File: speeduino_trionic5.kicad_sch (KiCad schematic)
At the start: 3 parts, among them U1 Olimex_STM32-407_Extension_He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

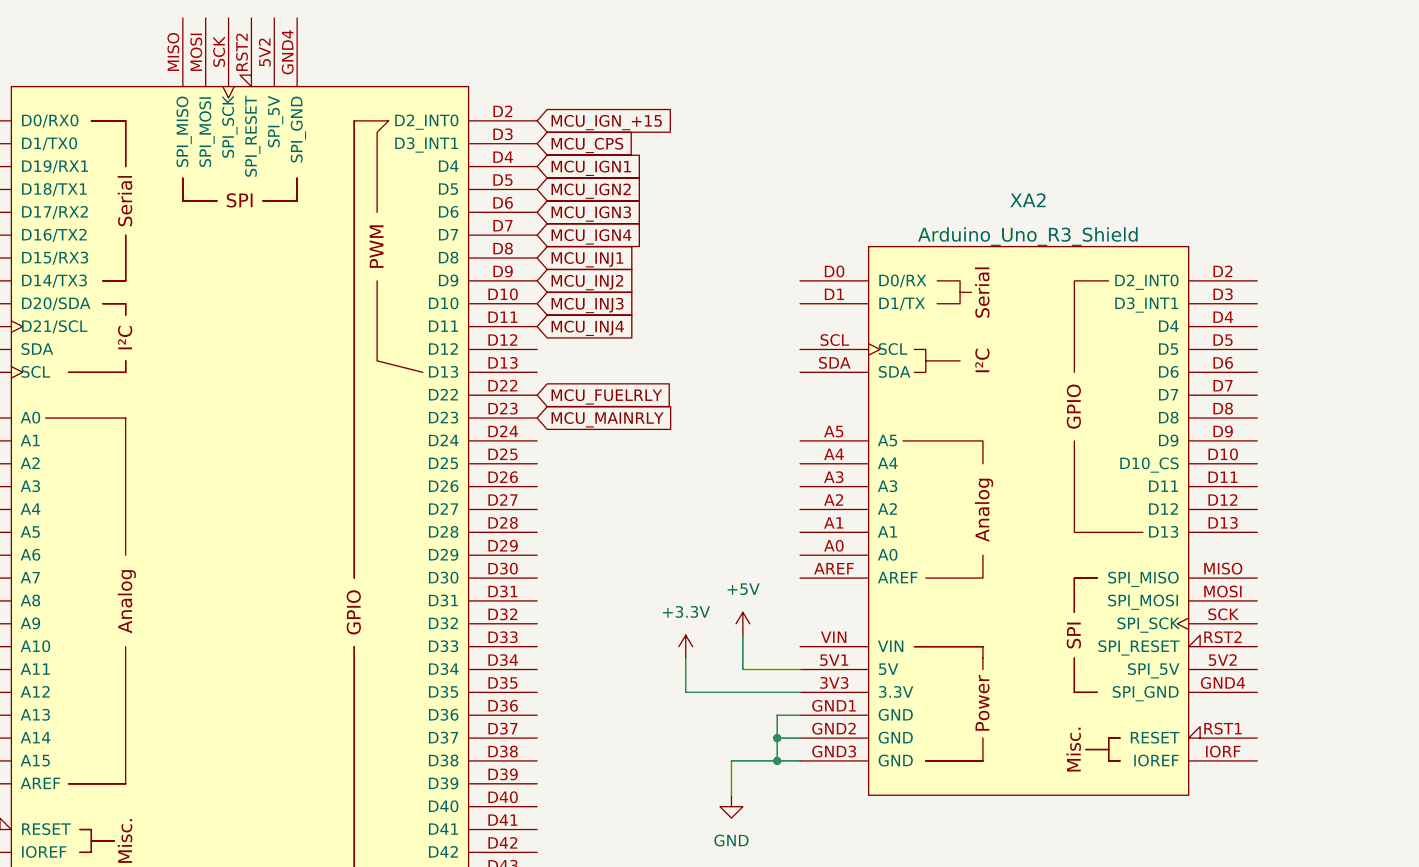
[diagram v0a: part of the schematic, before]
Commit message: Add stuff
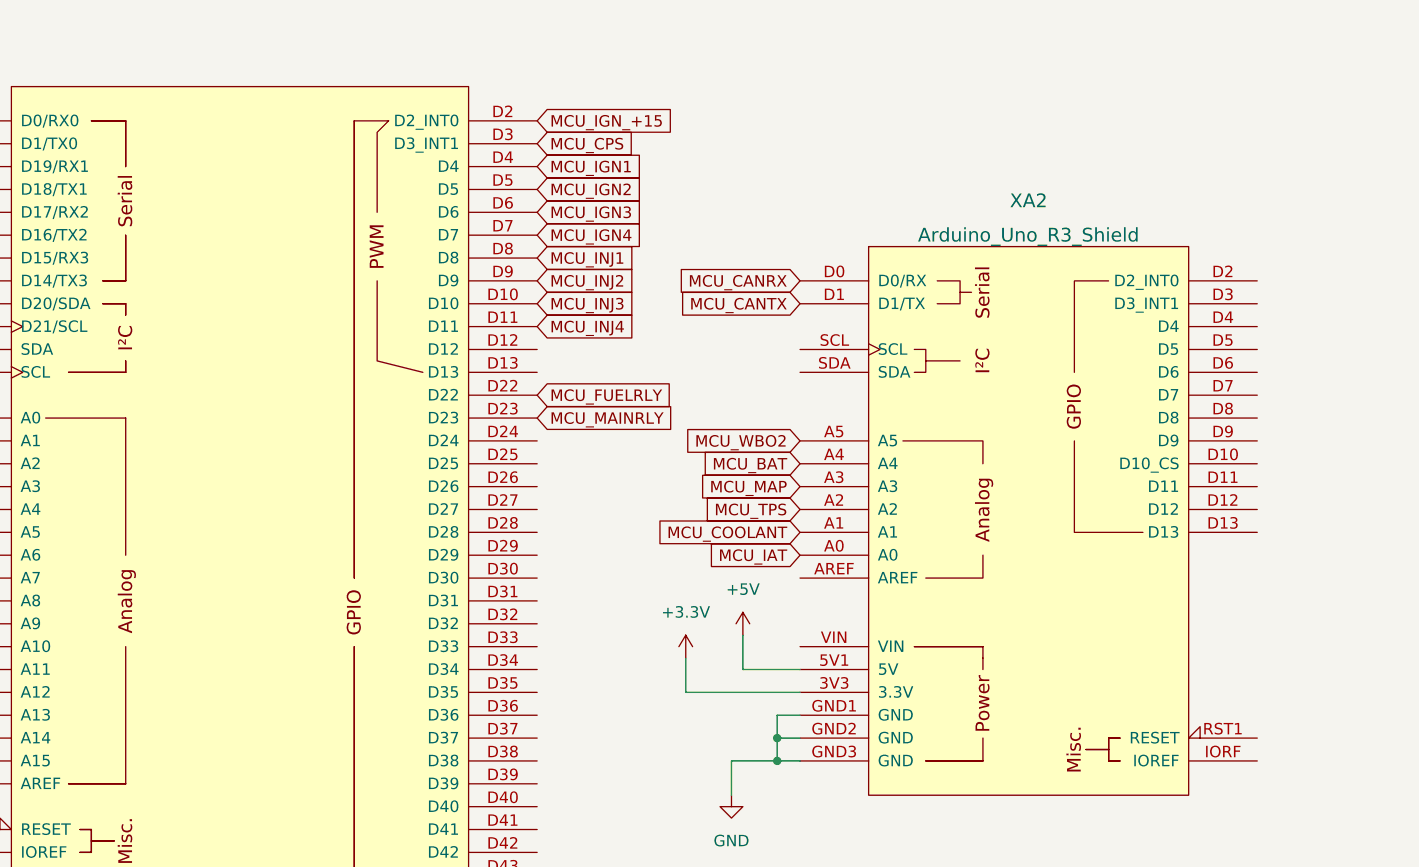
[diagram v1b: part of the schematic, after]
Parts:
- XA1: footprint PCM_arduino-library:Arduino_Mega2560_Shield -> arduino-library:Arduino_Mega2560_Shield
- XA2: footprint PCM_arduino-library:Arduino_Uno_R3_Shield -> arduino-library:Arduino_Uno_R3_Shield
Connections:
- net MCU_BAT: now also XA2.A4
- net MCU_COOLANT: now also XA2.A1
- net MCU_IAT: now also XA2.A0
- net MCU_MAP: now also XA2.A3
- net MCU_TPS: now also XA2.A2
- net MCU_WBO2: now also XA2.A5
- net MCU_CANRX: now reaches XA2.D0 (D0/RX)
- net MCU_CANTX: now reaches XA2.D1 (D1/TX)
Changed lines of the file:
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@@
     (stroke (width 0) (type default) (color 0 0 0 0))
   )
+  (global_label "MCU_MAP" (shape input) (at 129.54 76.2 180) (fields_autoplaced)
+    (effects (font (size 1.27 1.27)) (justify right))
+    (property "Intersheet References" "${INTERSHEET_REFS}" (id 0) (at 118.3863 76.1206 0)
+      (effects (font (size 1.27 1.27)) (justify right) hide)
+    )
+  )
+  (global_label "MCU_BAT" (shape input) (at 129.54 73.66 180) (fields_autoplaced)
+    (effects (font (size 1.27 1.27)) (justify right))
+    (property "Intersheet References" "${INTERSHEET_REFS}" (id 0) (at 118.8701 73.5806 0)
+      (effects (font (size 1.27 1.27)) (justify right) hide)
+    )
+  )
+  (global_label "MCU_CANTX" (shape input) (at 129.54 55.88 180) (fields_autoplaced)
+    (effects (font (size 1.27 1.27)) (justify right))
+    (property "Intersheet References" "${INTERSHEET_REFS}" (id 0) (at 116.3301 55.8006 0)
+      (effects (font (size 1.27 1.27)) (justify right) hide)
+    )
+  )
   (global_label "MCU_INJ3" (shape input) (at 100.33 55.88 0) (fields_autoplaced)
     (effects (font (size 1.27 1.27)) (justify left))
@@
     )
   )
+  (global_label "MCU_TPS" (shape input) (at 129.54 78.74 180) (fields_autoplaced)
+    (effects (font (size 1.27 1.27)) (justify right))
+    (property "Intersheet References" "${INTERSHEET_REFS}" (id 0) (at 118.7491 78.6606 0)
+      (effects (font (size 1.27 1.27)) (justify right) hide)
+    )
+  )
+  (global_label "MCU_CANRX" (shape input) (at 129.54 53.34 180) (fields_autoplaced)
+    (effects (font (size 1.27 1.27)) (justify right))
+    (property "Intersheet References" "${INTERSHEET_REFS}" (id 0) (at 116.0277 53.2606 0)
+      (effects (font (size 1.27 1.27)) (justify right) hide)
+    )
+  )
+  (global_label "MCU_IAT" (shape input) (at 129.54 83.82 180) (fields_autoplaced)
+    (effects (font (size 1.27 1.27)) (justify right))
+    (property "Intersheet References" "${INTERSHEET_REFS}" (id 0) (at 119.5353 83.7406 0)
+      (effects (font (size 1.27 1.27)) (justify right) hide)
+    )
+  )
   (global_label "MCU_INJ4" (shape input) (at 100.33 58.42 0) (fields_autoplaced)
     (effects (font (size 1.27 1.27)) (justify left))
@@
     )
   )
+  (global_label "MCU_WBO2" (shape input) (at 129.54 71.12 180) (fields_autoplaced)
+    (effects (font (size 1.27 1.27)) (justify right))
+    (property "Intersheet References" "${INTERSHEET_REFS}" (id 0) (at 116.9348 71.0406 0)
+      (effects (font (size 1.27 1.27)) (justify right) hide)
+    )
+  )
   (global_label "MCU_MAINRLY" (shape input) (at 100.33 68.58 0) (fields_autoplaced)
     (effects (font (size 1.27 1.27)) (justify left))
@@
     (property "Intersheet References" "${INTERSHEET_REFS}" (id 0) (at 112.0885 43.1006 0)
       (effects (font (size 1.27 1.27)) (justify left) hide)
+    )
+  )
+  (global_label "MCU_COOLANT" (shape input) (at 129.54 81.28 180) (fields_autoplaced)
+    (effects (font (size 1.27 1.27)) (justify right))
+    (property "Intersheet References" "${INTERSHEET_REFS}" (id 0) (at 113.8506 81.2006 0)
+      (effects (font (size 1.27 1.27)) (justify right) hide)
     )
   )
@@
       (effects (font (size 1.524 1.524)))
     )
-    (property "Footprint" "PCM_arduino-library:Arduino_Mega2560_Shield" (id 2) (at 67.31 163.83 0)
+    (property "Footprint" "arduino-library:Arduino_Mega2560_Shield" (id 2) (at 67.31 163.83 0)
       (effects (font (size 1.524 1.524)) hide)
     )
@@
     (pin "3V3")
     (pin "5V1")
-    (pin "5V2")
     (pin "5V3")
     (pin "5V4")
@@
     (pin "GND2")
     (pin "GND3")
-    (pin "GND4")
     (pin "GND5")
     (pin "GND6")
     (pin "IORF")
-    (pin "MISO")
-    (pin "MOSI")
     (pin "RST1")
-    (pin "RST2")
-    (pin "SCK")
     (pin "SCL")
     (pin "SDA")
@@
       (effects (font (size 1.524 1.524)))
     )
-    (property "Footprint" "PCM_arduino-library:Arduino_Uno_R3_Shield" (id 2) (at 154.94 118.11 0)
+    (property "Footprint" "arduino-library:Arduino_Uno_R3_Shield" (id 2) (at 154.94 118.11 0)
       (effects (font (size 1.524 1.524)) hide)
     )
@@
     (pin "3V3")
     (pin "5V1")
-    (pin "5V2")
     (pin "A0")
     (pin "A1")
@@
     (pin "GND2")
     (pin "GND3")
-    (pin "GND4")
     (pin "IORF")
-    (pin "MISO")
-    (pin "MOSI")
     (pin "RST1")
-    (pin "RST2")
-    (pin "SCK")
     (pin "SCL")
     (pin "SDA")
@@
       (reference "#PWR0160") (unit 1) (value "+3.3V") (footprint "")
     )
+    (path "/00000000-0000-0000-0000-00005cdc3535/69f1c3af-aba9-41f3-9359-5cd63804d515"
+      (reference "#PWR0161") (unit 1) (value "GND") (footprint "")
+    )
+    (path "/00000000-0000-0000-0000-00005cdc3535/baa221e7-3e5a-4913-9d1c-062714ac06ad"
+      (reference "#PWR0162") (unit 1) (value "+3.3V") (footprint "")
+    )
     (path "/00000000-0000-0000-0000-00005cd18d89/46ccbee1-4e2a-4bf8-8e1f-6e0ffec1a5d0"
       (reference "C1") (unit 1) (value "1nF") (footprint "Capacitor_SMD:C_0603_1608Metric")
@@
       (reference "U3") (unit 1) (value "LM1815") (footprint "Package_SO:SOIC-14_3.9x8.7mm_P1.27mm")
     )
+    (path "/00000000-0000-0000-0000-00005cdc3535/50a4570c-9d6b-4685-87a8-34989ca07b37"
+      (reference "U4") (unit 1) (value "TCAN330") (footprint "Package_TO_SOT_SMD:SOT-23-8")
+    )
     (path "/00000000-0000-0000-0000-00005cd18ec3/00000000-0000-0000-0000-00005cfc6620"
       (reference "U8") (unit 1) (value "LM2940S-5.0/NOPB") (footprint "Package_TO_SOT_SMD:SOT-223")
     )
     (path "/23c553c0-474e-48ea-9717-5d046a86dbed"
-      (reference "XA1") (unit 1) (value "Arduino_Mega2560_Shield") (footprint "PCM_arduino-library:Arduino_Mega2560_Shield")
+      (reference "XA1") (unit 1) (value "Arduino_Mega2560_Shield") (footprint "arduino-library:Arduino_Mega2560_Shield")
     )
     (path "/3ae2ecba-da25-4af2-bfd2-c505596d3e7f"
-      (reference "XA2") (unit 1) (value "Arduino_Uno_R3_Shield") (footprint "PCM_arduino-library:Arduino_Uno_R3_Shield")
-    )
-  )
+      (reference "XA2") (unit 1) (value "Arduino_Uno_R3_Shield") (footprint "arduino-library:Arduino_Uno_R3_Shield")
+    )
+  )
